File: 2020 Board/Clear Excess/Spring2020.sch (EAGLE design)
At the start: 30 parts

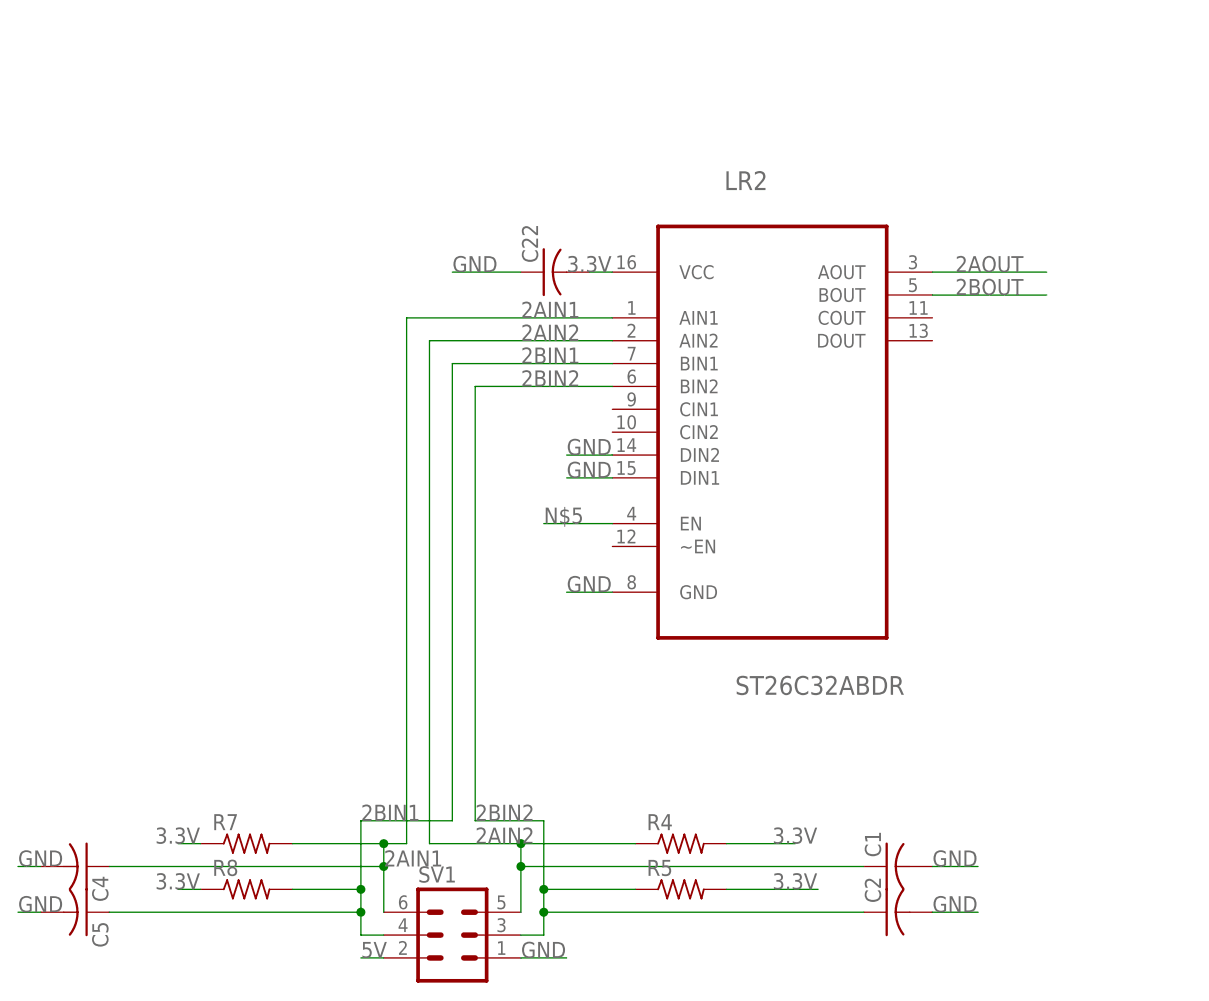
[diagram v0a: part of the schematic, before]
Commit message: Some more cleanup
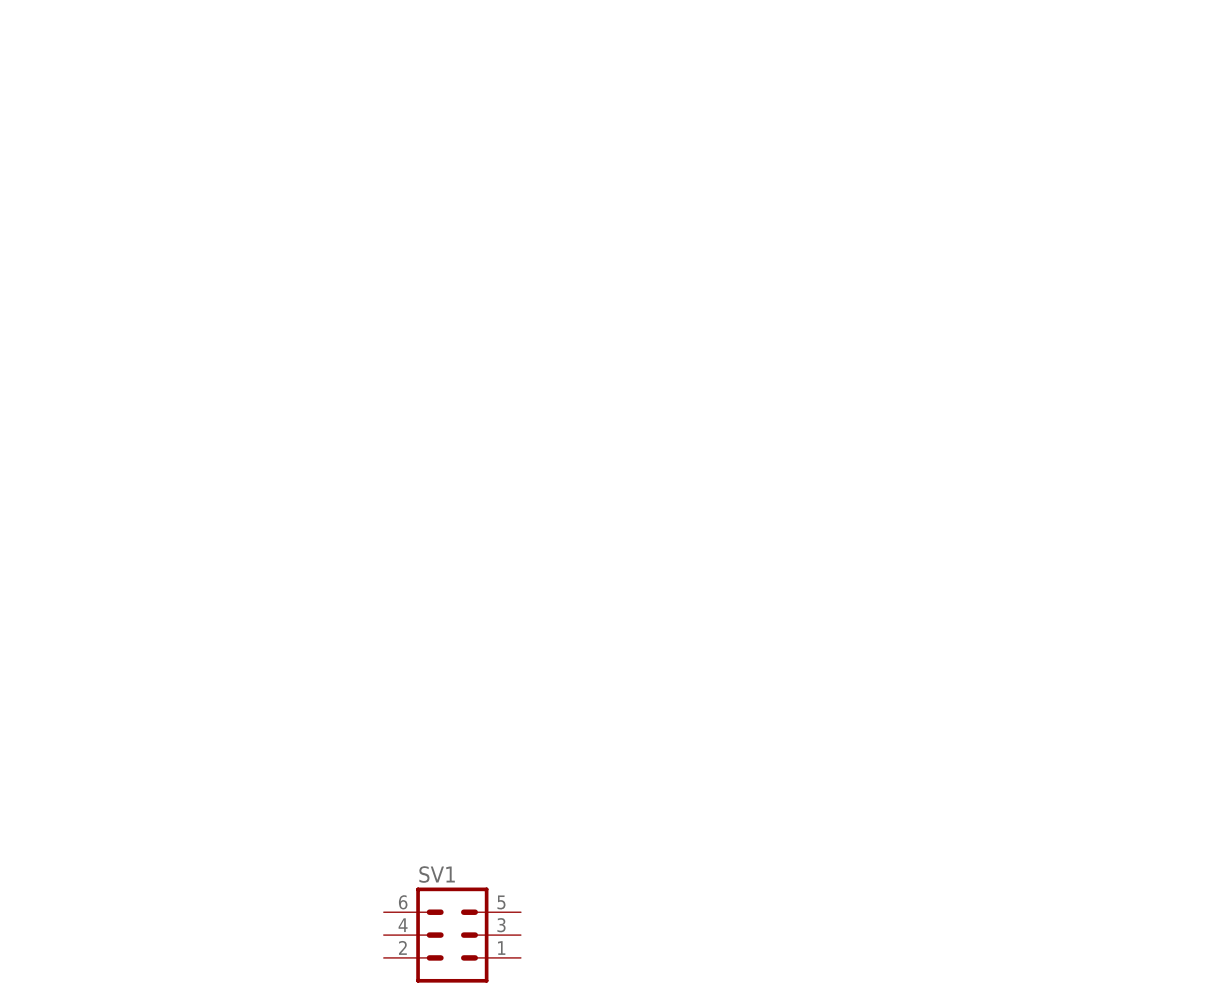
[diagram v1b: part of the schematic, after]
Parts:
- removed C1, C2, C4, C5: (no value), resistor:C-US025-025X050
- removed C22: (no value), resistor:C-US025-050X050
- removed LR2: ST26C32ABDR, BikeTeamLR:ST26C32ABDR
- removed R4, R5, R7, R8: (no value), resistor:R-US_0613/15
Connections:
- removed net 2AIN1: C4.1, LR2.AIN1, R7.2, SV1.6
- removed net 2AIN2: C1.1, LR2.AIN2, R4.1, SV1.5
- removed net 2AOUT: LR2.AOUT
- removed net 2BIN1: C5.1, LR2.BIN1, R8.2, SV1.4
- removed net 2BIN2: C2.1, LR2.BIN2, R5.1, SV1.3
- removed net 2BOUT: LR2.BOUT
- removed net N$2: C22.1
- removed net N$5: LR2.EN
- net 3.3V: no longer C22.2, LR2.VCC, R4.2, R5.2, R7.1, R8.1
- net 5V: no longer SV1.2
- net GND: no longer C1.2, C2.2, C4.2, C5.2, LR2.DIN1, LR2.DIN2, LR2.GND, SV1.1

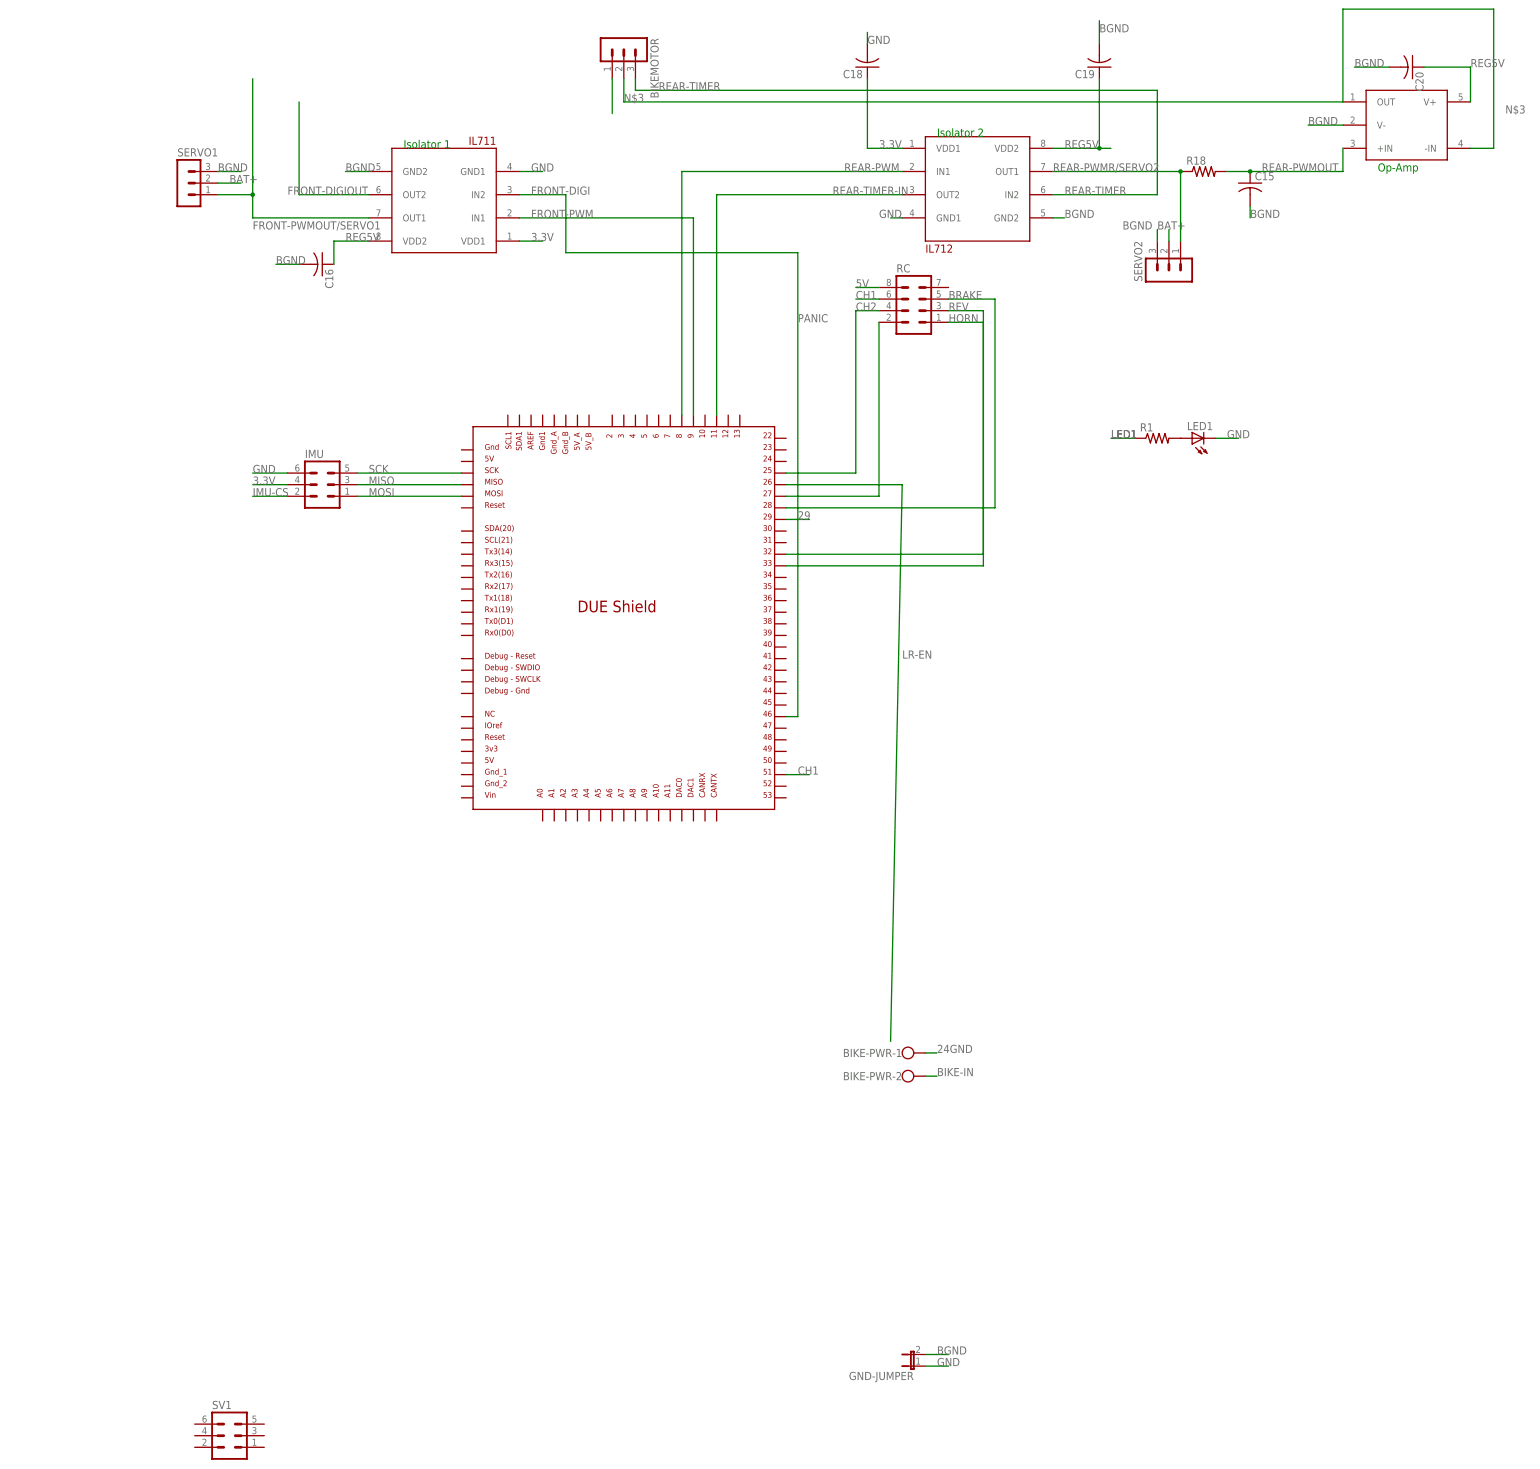
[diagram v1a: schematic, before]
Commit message: Final Cleaning of Bike
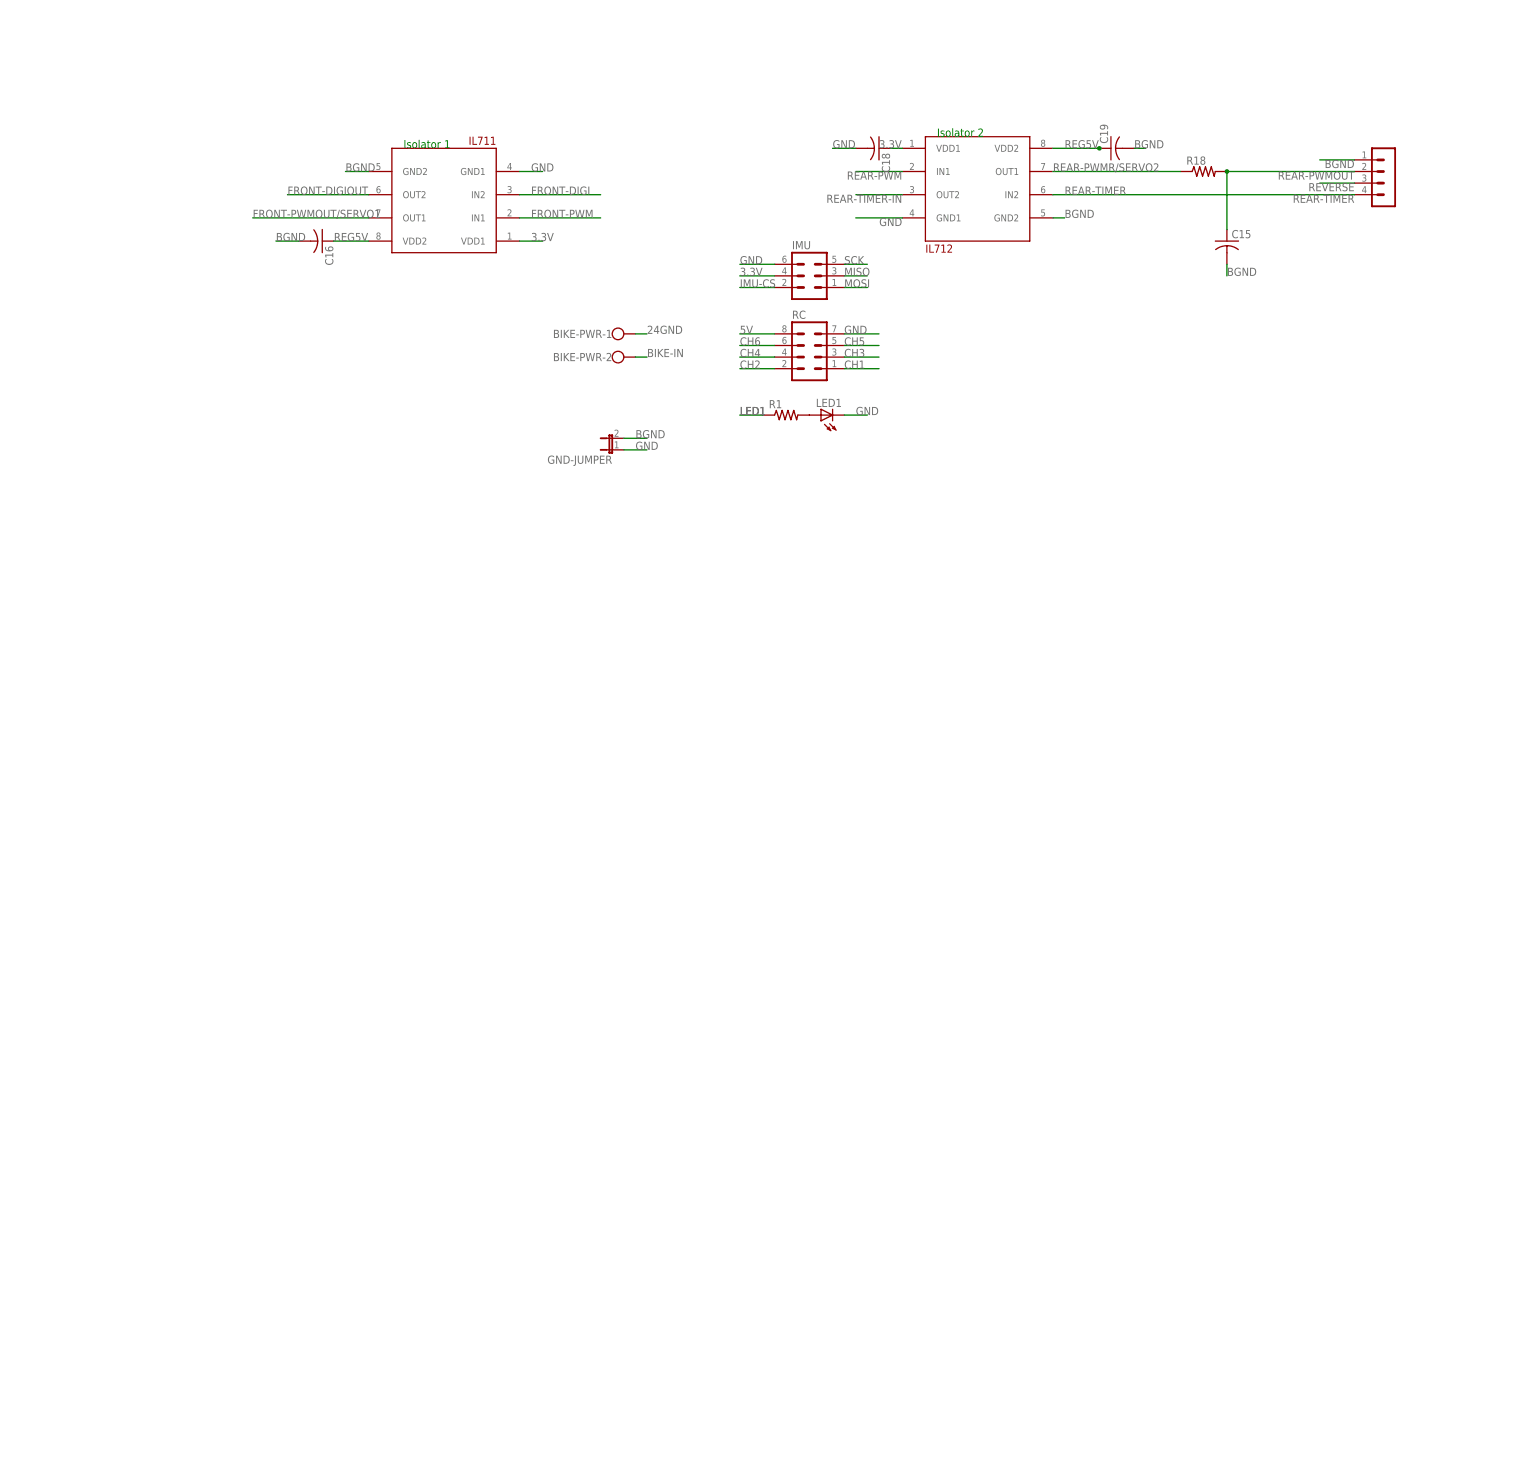
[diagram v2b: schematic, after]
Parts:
- removed BIKEMOTOR, SERVO1, SERVO2: (no value), con-lstb:MA03-1
- removed C20: (no value), resistor:C-US025-050X050
- removed OP-AMP: OPAMP, Spring2016opamp:OPAMP
- removed SV1: (no value), con-lstb:MA03-2
- removed U$1: DUE(NORMAL), DUElib130425:DUE(NORMAL)
- added REAR-MOTOR: (no value), con-lstb:MA04-1
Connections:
- removed net 29: U$1.29
- removed net BAT+: SERVO1.2, SERVO2.2
- removed net BRAKE: RC.5, U$1.28
- removed net HORN: RC.1, U$1.32
- removed net LR-EN: U$1.26
- removed net N$3: BIKEMOTOR.2, OP-AMP.-IN, OP-AMP.OUT
- removed net N$4: BIKEMOTOR.1
- removed net PANIC: RC.2, U$1.27
- removed net REV: RC.3, U$1.33
- new net CH3: RC.3
- new net CH4: RC.4
- new net CH5: RC.5
- new net CH6: RC.6
- new net REVERSE: REAR-MOTOR.3
- net BGND: now also REAR-MOTOR.1; no longer C20.2, OP-AMP.V-, SERVO1.3, SERVO2.3
- net CH1: now also RC.1; no longer RC.6, U$1.51
- net CH2: now also RC.2; no longer RC.4, U$1.25
- net FRONT-DIGI: no longer U$1.46
- net FRONT-PWM: no longer U$1.9
- net FRONT-PWMOUT/SERVO1: no longer SERVO1.1
- net GND: now also RC.7
- net MISO: no longer U$1.MISO_ICSP
- net MOSI: no longer U$1.MOSI_ICSP
- net REAR-PWM: no longer U$1.8
- net REAR-PWMOUT: now also REAR-MOTOR.2; no longer OP-AMP.+IN
- net REAR-PWMR/SERVO2: no longer SERVO2.1
- net REAR-TIMER: now also REAR-MOTOR.4; no longer BIKEMOTOR.3
- net REAR-TIMER-IN: no longer U$1.11
- net REG5V: no longer C20.1, OP-AMP.V+
- net SCK: no longer U$1.SCK_ICSP
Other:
- note removed: "Op-Amp"
- moved on the sheet: BIKE-PWR-1, BIKE-PWR-2, C15, C16, C18, C19, GND-JUMPER, IMU, LED1, R1, RC
